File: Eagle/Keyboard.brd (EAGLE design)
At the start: 100 x 80 mm, 104 parts

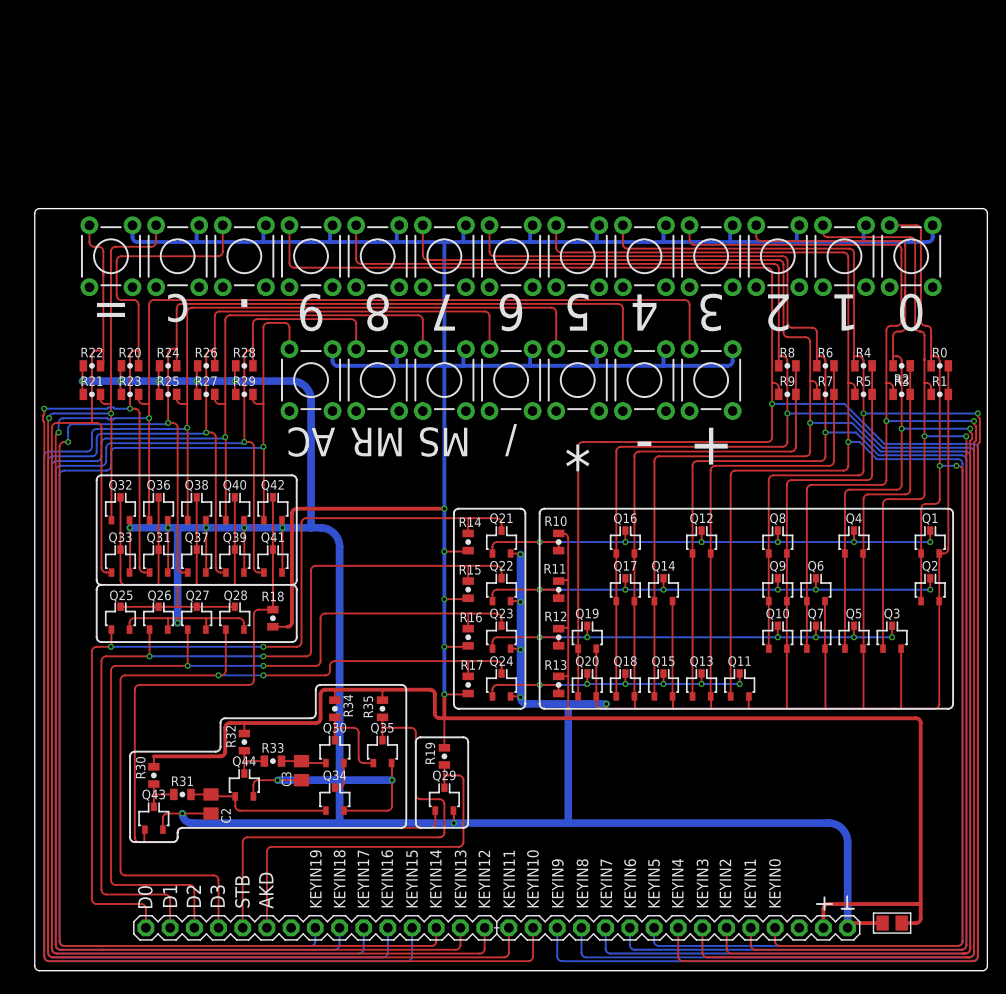
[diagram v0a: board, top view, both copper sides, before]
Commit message: Updated with pcb template
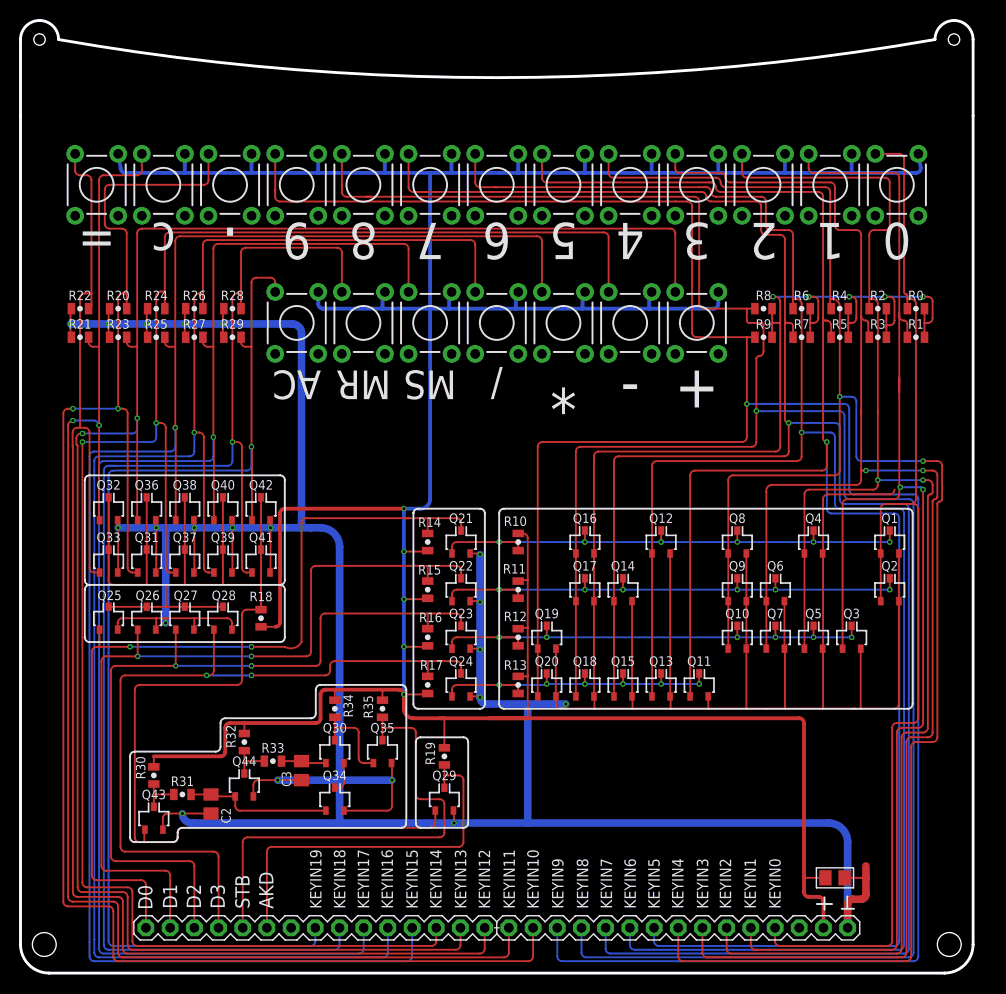
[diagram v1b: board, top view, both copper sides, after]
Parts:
- moved C1 7.65 mm to (84.0, 9.75), turned to 0 degrees
- moved S0 7.65 mm to (90.5, 82.5)
- moved S1 7.65 mm to (83.5, 82.5)
- moved S10 7.65 mm to (20.5, 82.5)
- moved S11 7.65 mm to (13.5, 82.5)
- moved S12 7.65 mm to (6.50, 82.5)
- moved S2 7.65 mm to (76.5, 82.5)
- moved S3 7.65 mm to (69.5, 82.5)
- moved S4 7.65 mm to (62.5, 82.5)
- moved S5 7.65 mm to (55.5, 82.5)
- moved S6 7.65 mm to (48.5, 82.5)
- moved S7 7.65 mm to (41.5, 82.5)
- moved S8 7.65 mm to (34.5, 82.5)
- moved S9 7.65 mm to (27.5, 82.5)
- moved R0 6.50 mm to (92.5, 69.5)
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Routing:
- net GND: track 617.9 -> 599.2 mm, vias 20 -> 25
- net VCC: track 406.9 -> 394.7 mm
- net KEYIN9: track 246.0 -> 254.7 mm
- net KEYIN19: track 128.6 -> 120.7 mm
- net KEYIN3: track 174.1 -> 167.0 mm
- net D0: track 95.2 -> 90.7 mm
- net D3: track 84.7 -> 80.4 mm
- net D2: track 87.7 -> 83.4 mm
- net D1: track 91.2 -> 86.9 mm
- net KEYIN2: track 159.2 -> 155.2 mm
- net KEYIN0: track 121.3 -> 117.8 mm, vias 2 -> 0
- net KEYIN18: track 148.8 -> 145.9 mm
- net KEYIN4: track 183.3 -> 186.1 mm
- net KEYIN13: track 196.0 -> 198.1 mm
- net KEYIN17: track 153.5 -> 151.4 mm
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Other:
- board size 100 x 80 mm -> 100 x 100 mm
- board text added: "Xxxxxx yyyyy rev1"
- board text removed: "Keyboard decoder Rev1"
